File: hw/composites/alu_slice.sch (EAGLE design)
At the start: 13 parts, among them CON2 GENERIC-2X10

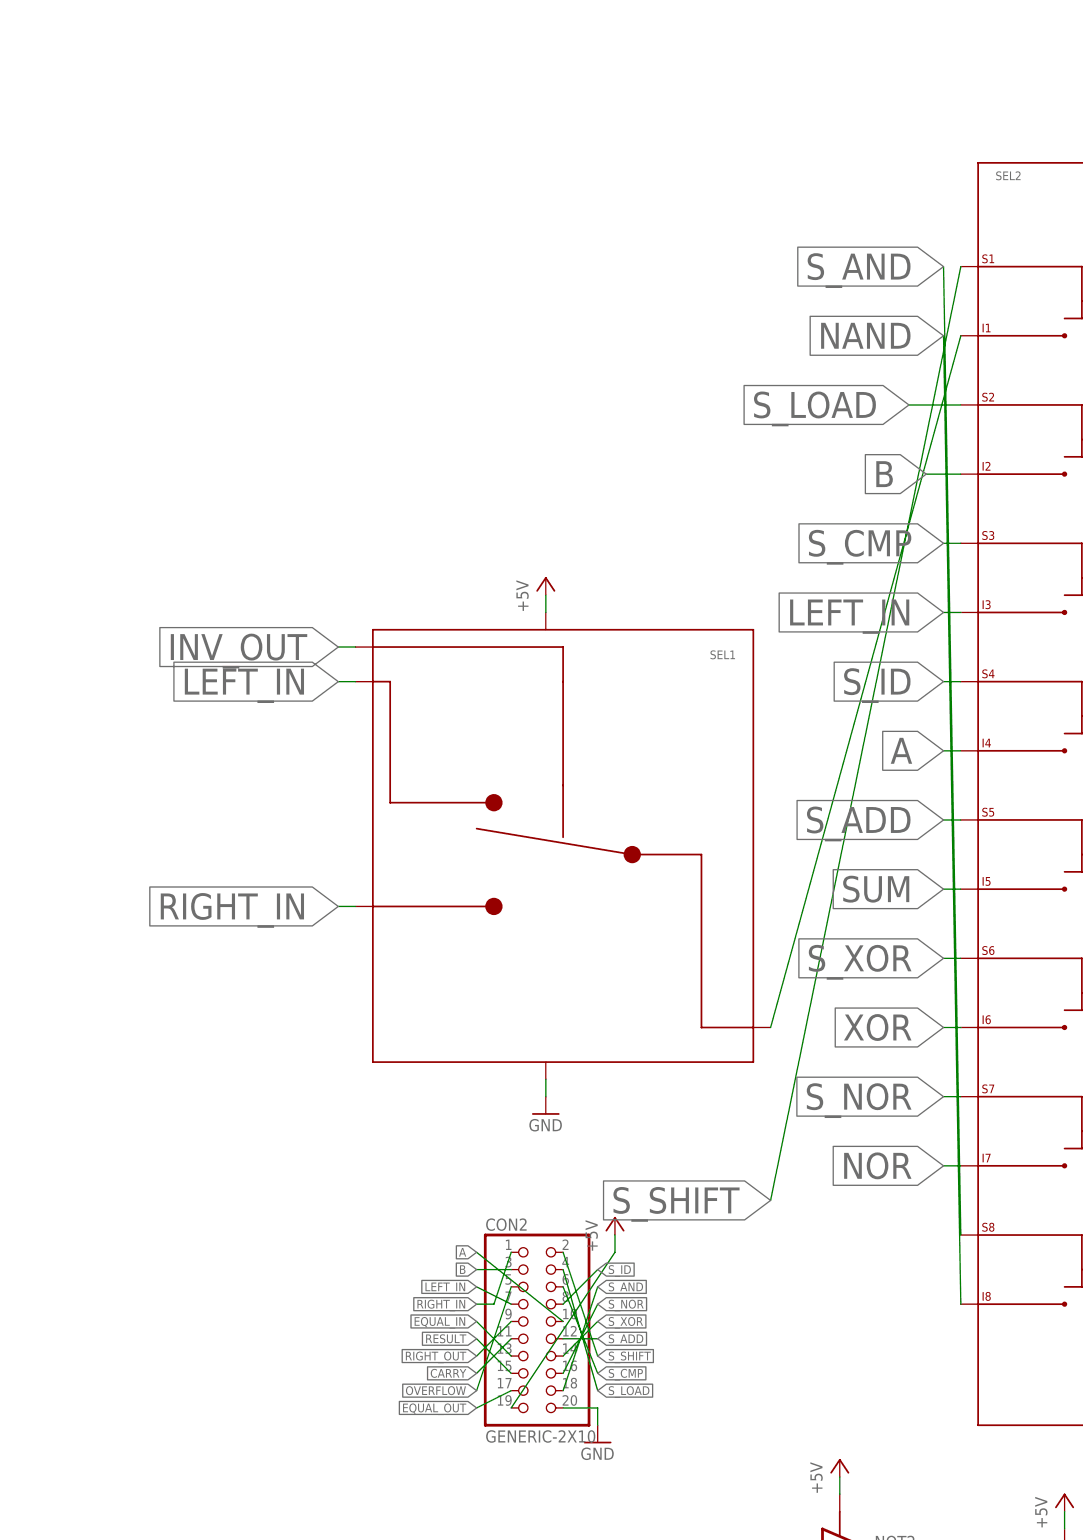
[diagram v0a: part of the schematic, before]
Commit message: Basic cleanups
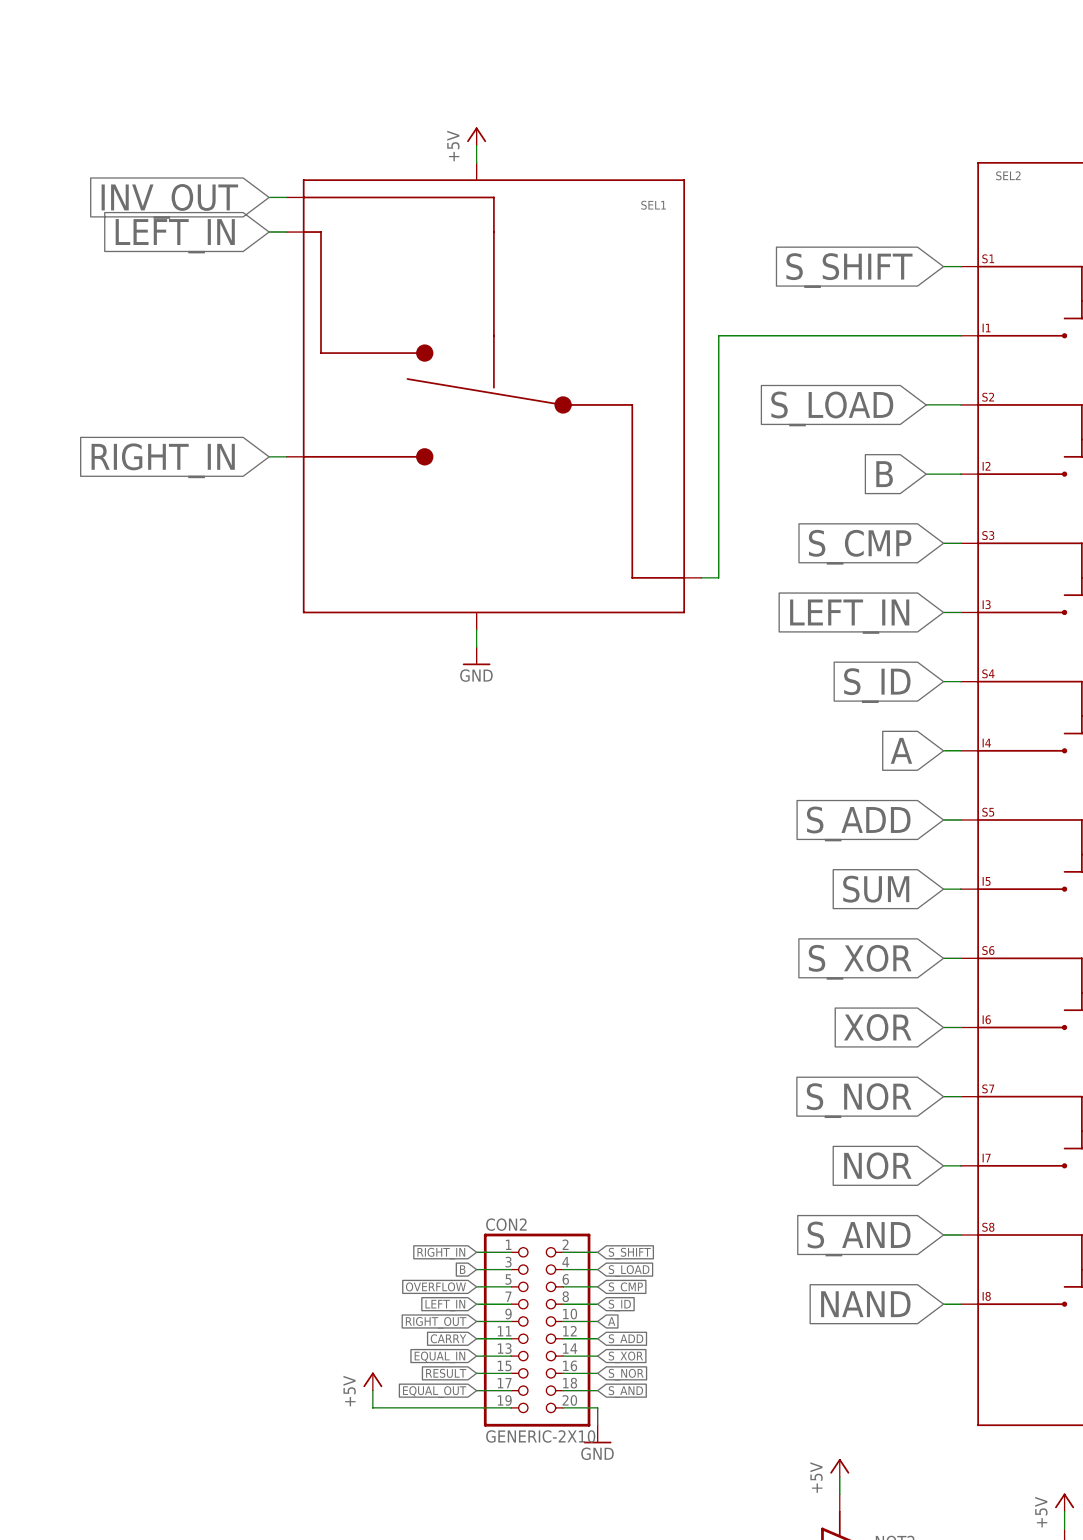
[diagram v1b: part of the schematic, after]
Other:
- moved on the sheet: SEL1
